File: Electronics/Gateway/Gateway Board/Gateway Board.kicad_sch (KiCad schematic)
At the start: 6 parts

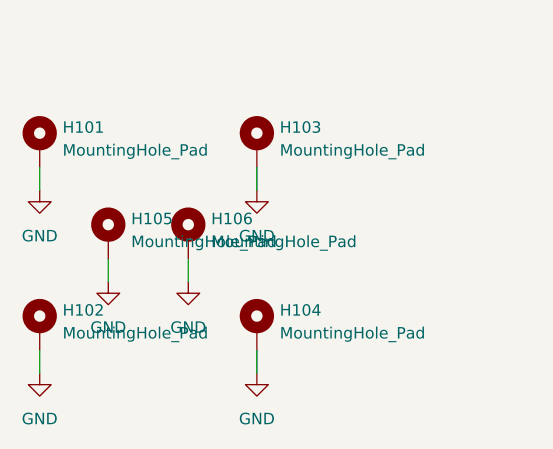
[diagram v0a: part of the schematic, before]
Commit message: All boards done
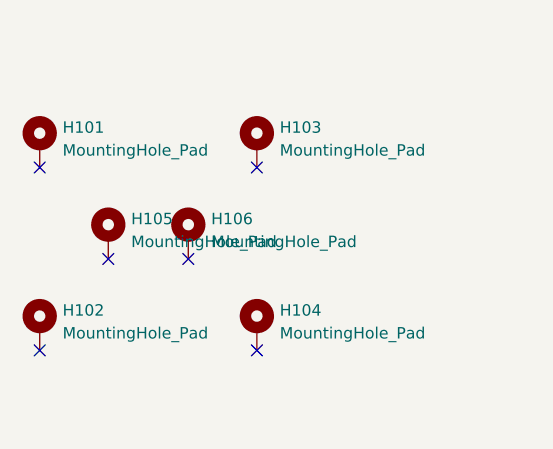
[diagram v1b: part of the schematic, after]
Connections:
- removed net GND: H101.1, H102.1, H103.1, H104.1, H105.1, H106.1
- no-connect marks 0 -> 6
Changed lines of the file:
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@@
 (kicad_sch (version 20230121) (generator eeschema)
   (paper "A5")
-  (wire (pts (xy 40.64 116.84) (xy 40.64 114.3))
-    (stroke (width 0) (type default))
-  )
-  (wire (pts (xy 33.02 106.68) (xy 33.02 104.14))
-    (stroke (width 0) (type default))
-  )
-  (wire (pts (xy 49.53 116.84) (xy 49.53 114.3))
-    (stroke (width 0) (type default))
-  )
-  (wire (pts (xy 57.15 106.68) (xy 57.15 104.14))
-    (stroke (width 0) (type default))
-  )
-  (wire (pts (xy 33.02 127) (xy 33.02 124.46))
-    (stroke (width 0) (type default))
-  )
-  (wire (pts (xy 57.15 127) (xy 57.15 124.46))
-    (stroke (width 0) (type default))
-  )
+  (no_connect (at 33.02 104.14))
+  (no_connect (at 49.53 114.3))
+  (no_connect (at 57.15 124.46))
+  (no_connect (at 40.64 114.3))
+  (no_connect (at 33.02 124.46))
+  (no_connect (at 57.15 104.14))
   (symbol (lib_id "Mechanical:MountingHole_Pad") (at 57.15 121.92 0) (unit 1)
     (in_bom yes) (on_board yes) (dnp no) (fields_autoplaced)
@@
         (path "/d8843e0a-fd8a-4193-ba57-f0164156e030"
           (reference "H4") (unit 1)
-        )
-      )
-    )
-  )
-  (symbol (lib_id "power:GND") (at 57.15 127 0) (unit 1)
-    (in_bom yes) (on_board yes) (dnp no) (fields_autoplaced)
-    (property "Reference" "#PWR0104" (at 57.15 133.35 0)
-      (effects (font (size 1.27 1.27)) hide)
-    )
-    (property "Value" "GND" (at 57.15 132.08 0)
-      (effects (font (size 1.27 1.27)))
-    )
-    (property "Footprint" "" (at 57.15 127 0)
-      (effects (font (size 1.27 1.27)) hide)
-    )
-    (property "Datasheet" "" (at 57.15 127 0)
-      (effects (font (size 1.27 1.27)) hide)
-    )
-    (pin "1")
-    (instances
-      (project "Gateway Board"
-        (path "/5318664d-e328-4e84-a383-7318275dc447"
-          (reference "#PWR0104") (unit 1)
-        )
-      )
-      (project "Power Board"
-        (path "/d8843e0a-fd8a-4193-ba57-f0164156e030"
-          (reference "#PWR04") (unit 1)
         )
       )
@@
     )
   )
-  (symbol (lib_id "power:GND") (at 57.15 106.68 0) (unit 1)
-    (in_bom yes) (on_board yes) (dnp no) (fields_autoplaced)
-    (property "Reference" "#PWR0103" (at 57.15 113.03 0)
-      (effects (font (size 1.27 1.27)) hide)
-    )
-    (property "Value" "GND" (at 57.15 111.76 0)
-      (effects (font (size 1.27 1.27)))
-    )
-    (property "Footprint" "" (at 57.15 106.68 0)
-      (effects (font (size 1.27 1.27)) hide)
-    )
-    (property "Datasheet" "" (at 57.15 106.68 0)
-      (effects (font (size 1.27 1.27)) hide)
-    )
-    (pin "1")
-    (instances
-      (project "Gateway Board"
-        (path "/5318664d-e328-4e84-a383-7318275dc447"
-          (reference "#PWR0103") (unit 1)
-        )
-      )
-      (project "Power Board"
-        (path "/d8843e0a-fd8a-4193-ba57-f0164156e030"
-          (reference "#PWR03") (unit 1)
-        )
-      )
-    )
-  )
-  (symbol (lib_id "power:GND") (at 40.64 116.84 0) (unit 1)
-    (in_bom yes) (on_board yes) (dnp no) (fields_autoplaced)
-    (property "Reference" "#PWR0105" (at 40.64 123.19 0)
-      (effects (font (size 1.27 1.27)) hide)
-    )
-    (property "Value" "GND" (at 40.64 121.92 0)
-      (effects (font (size 1.27 1.27)))
-    )
-    (property "Footprint" "" (at 40.64 116.84 0)
-      (effects (font (size 1.27 1.27)) hide)
-    )
-    (property "Datasheet" "" (at 40.64 116.84 0)
-      (effects (font (size 1.27 1.27)) hide)
-    )
-    (pin "1")
-    (instances
-      (project "Gateway Board"
-        (path "/5318664d-e328-4e84-a383-7318275dc447"
-          (reference "#PWR0105") (unit 1)
-        )
-      )
-      (project "Power Board"
-        (path "/d8843e0a-fd8a-4193-ba57-f0164156e030"
-          (reference "#PWR02") (unit 1)
-        )
-      )
-    )
-  )
   (symbol (lib_id "Mechanical:MountingHole_Pad") (at 57.15 101.6 0) (unit 1)
     (in_bom yes) (on_board yes) (dnp no) (fields_autoplaced)
@@
         (path "/d8843e0a-fd8a-4193-ba57-f0164156e030"
           (reference "H3") (unit 1)
-        )
-      )
-    )
-  )
-  (symbol (lib_id "power:GND") (at 49.53 116.84 0) (unit 1)
-    (in_bom yes) (on_board yes) (dnp no) (fields_autoplaced)
-    (property "Reference" "#PWR0106" (at 49.53 123.19 0)
-      (effects (font (size 1.27 1.27)) hide)
-    )
-    (property "Value" "GND" (at 49.53 121.92 0)
-      (effects (font (size 1.27 1.27)))
-    )
-    (property "Footprint" "" (at 49.53 116.84 0)
-      (effects (font (size 1.27 1.27)) hide)
-    )
-    (property "Datasheet" "" (at 49.53 116.84 0)
-      (effects (font (size 1.27 1.27)) hide)
-    )
-    (pin "1")
-    (instances
-      (project "Gateway Board"
-        (path "/5318664d-e328-4e84-a383-7318275dc447"
-          (reference "#PWR0106") (unit 1)
-        )
-      )
-      (project "Power Board"
-        (path "/d8843e0a-fd8a-4193-ba57-f0164156e030"
-          (reference "#PWR02") (unit 1)
         )
       )
@@
         )
       )
-    )
-  )
-  (symbol (lib_id "power:GND") (at 33.02 106.68 0) (unit 1)
-    (in_bom yes) (on_board yes) (dnp no) (fields_autoplaced)
-    (property "Reference" "#PWR0101" (at 33.02 113.03 0)
-      (effects (font (size 1.27 1.27)) hide)
-    )
-    (property "Value" "GND" (at 33.02 111.76 0)
-      (effects (font (size 1.27 1.27)))
-    )
-    (property "Footprint" "" (at 33.02 106.68 0)
-      (effects (font (size 1.27 1.27)) hide)
-    )
-    (property "Datasheet" "" (at 33.02 106.68 0)
-      (effects (font (size 1.27 1.27)) hide)
-    )
-    (pin "1")
-    (instances
-      (project "Gateway Board"
-        (path "/5318664d-e328-4e84-a383-7318275dc447"
-          (reference "#PWR0101") (unit 1)
-        )
-      )
-      (project "Power Board"
-        (path "/d8843e0a-fd8a-4193-ba57-f0164156e030"
-          (reference "#PWR01") (unit 1)
-        )
-      )
-    )
-  )
-  (symbol (lib_id "power:GND") (at 33.02 127 0) (unit 1)
-    (in_bom yes) (on_board yes) (dnp no) (fields_autoplaced)
-    (property "Reference" "#PWR0102" (at 33.02 133.35 0)
-      (effects (font (size 1.27 1.27)) hide)
-    )
-    (property "Value" "GND" (at 33.02 132.08 0)
-      (effects (font (size 1.27 1.27)))
-    )
-    (property "Footprint" "" (at 33.02 127 0)
-      (effects (font (size 1.27 1.27)) hide)
-    )
-    (property "Datasheet" "" (at 33.02 127 0)
-      (effects (font (size 1.27 1.27)) hide)
-    )
-    (pin "1")
-    (instances
-      (project "Gateway Board"
-        (path "/5318664d-e328-4e84-a383-7318275dc447"
-          (reference "#PWR0102") (unit 1)
-        )
-      )
-      (project "Power Board"
-        (path "/d8843e0a-fd8a-4193-ba57-f0164156e030"
-          (reference "#PWR02") (unit 1)
-        )
-      )
